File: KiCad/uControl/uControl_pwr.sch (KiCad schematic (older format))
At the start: 25 parts, among them P10 12V, Q1 FDN340P, U1 LP2985-33DBVR, U3 NCP1117ST50T3G, U5 LM358N

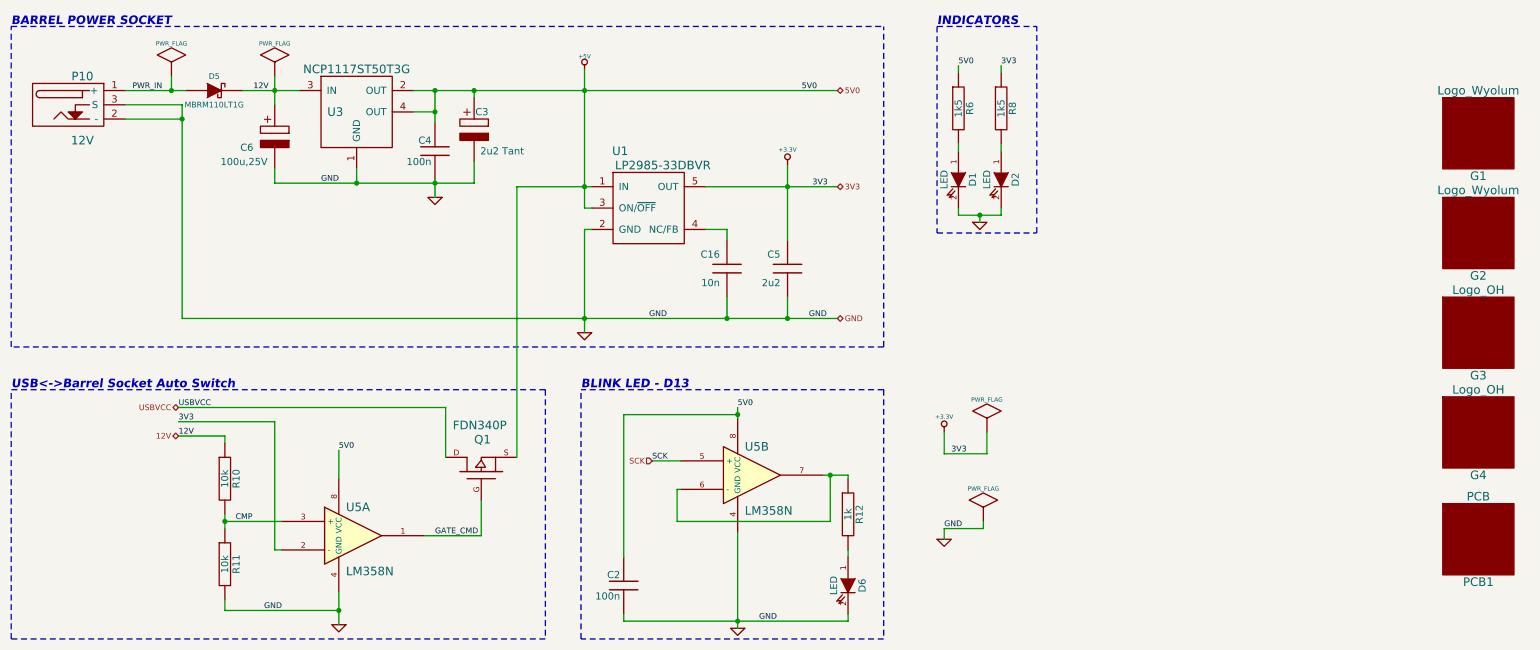
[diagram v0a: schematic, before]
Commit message: uControl some minor edits to schematic
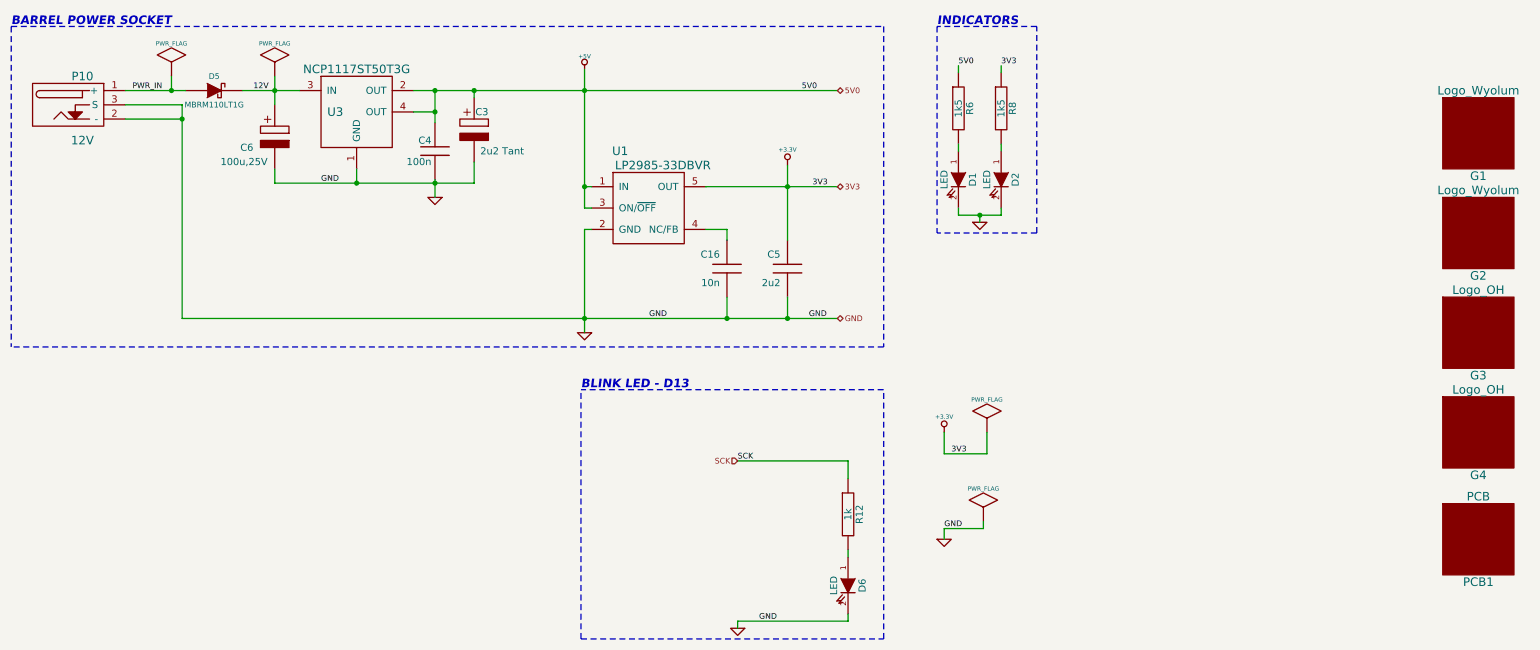
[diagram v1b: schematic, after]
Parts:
- removed C2: 100n, c_0805, symbol C
- removed Q1: FDN340P, SOT23-3, symbol MOSFET_P
- removed R10, R11: 10k, r_0805, symbol R
- removed U5: LM358N, SO8E, symbol LM358N
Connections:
- net SCK: now also R12.1
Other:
- note removed: "USB<->Barrel Socket Auto Switch"
